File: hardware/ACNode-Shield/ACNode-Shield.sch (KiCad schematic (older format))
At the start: 15 parts, among them J1 MICRO_SD_HINGE, P1 CONN_NFC, P2 CONN_RELAY, P3 CONN_RGB_LED, P4 CONN_X6, P5 CONN_X7, P6 CONN_WS2812, Q1 PN2222A, SW1 SW_RST, SW2 SW_BTN, U1 SRD-05VDC-SL-C, U2 WS2812B

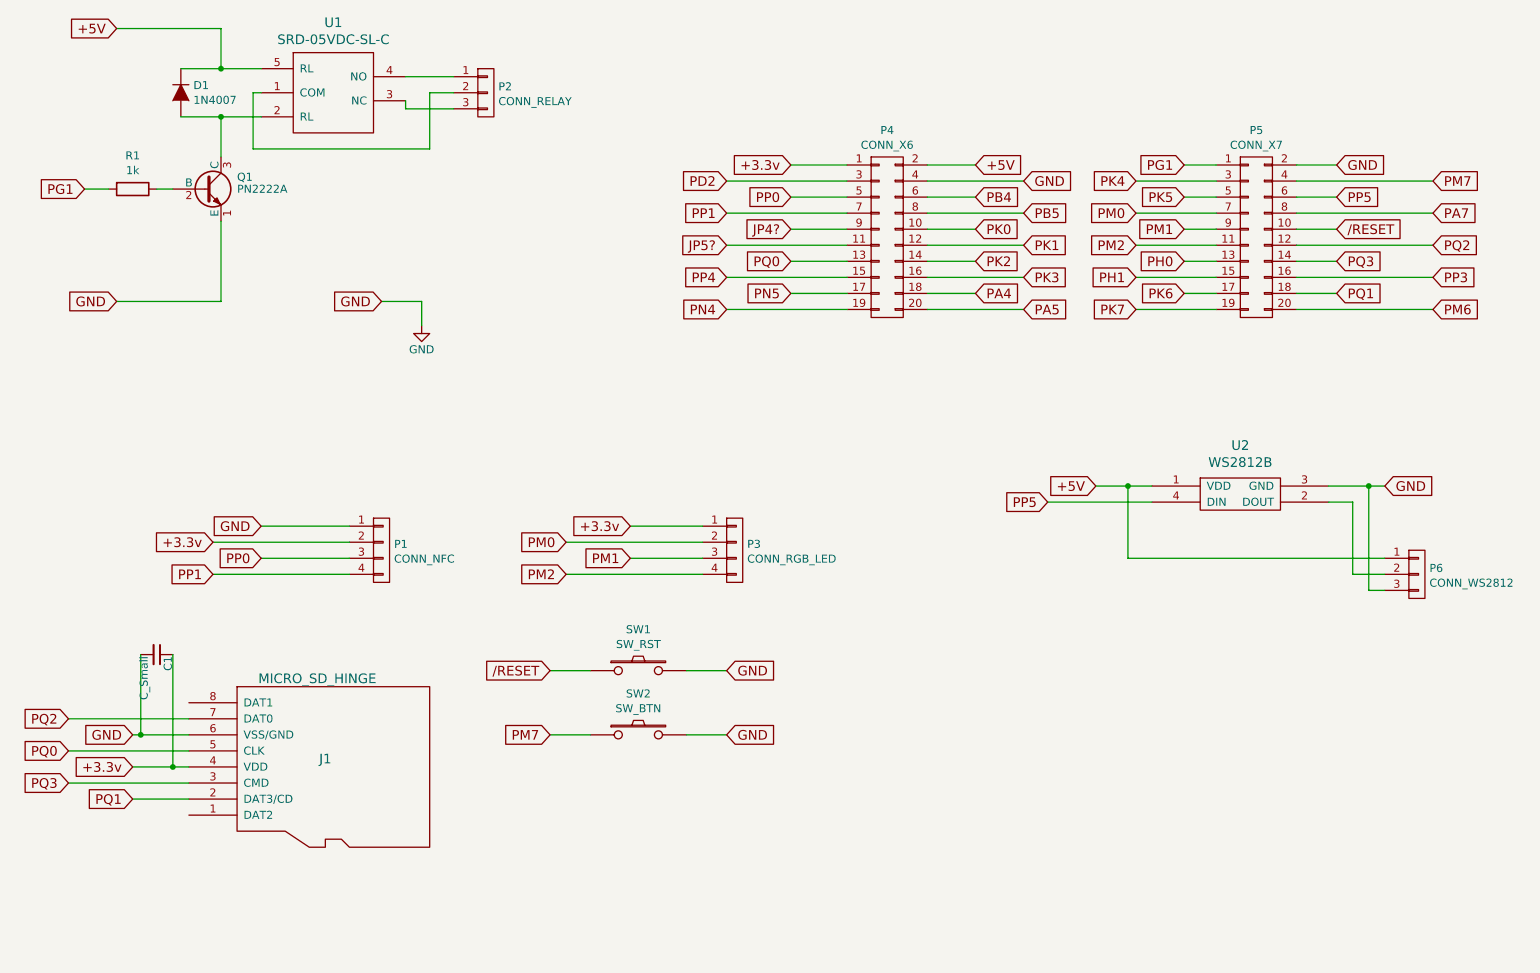
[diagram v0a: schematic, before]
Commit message: Rev 2 off to the fab
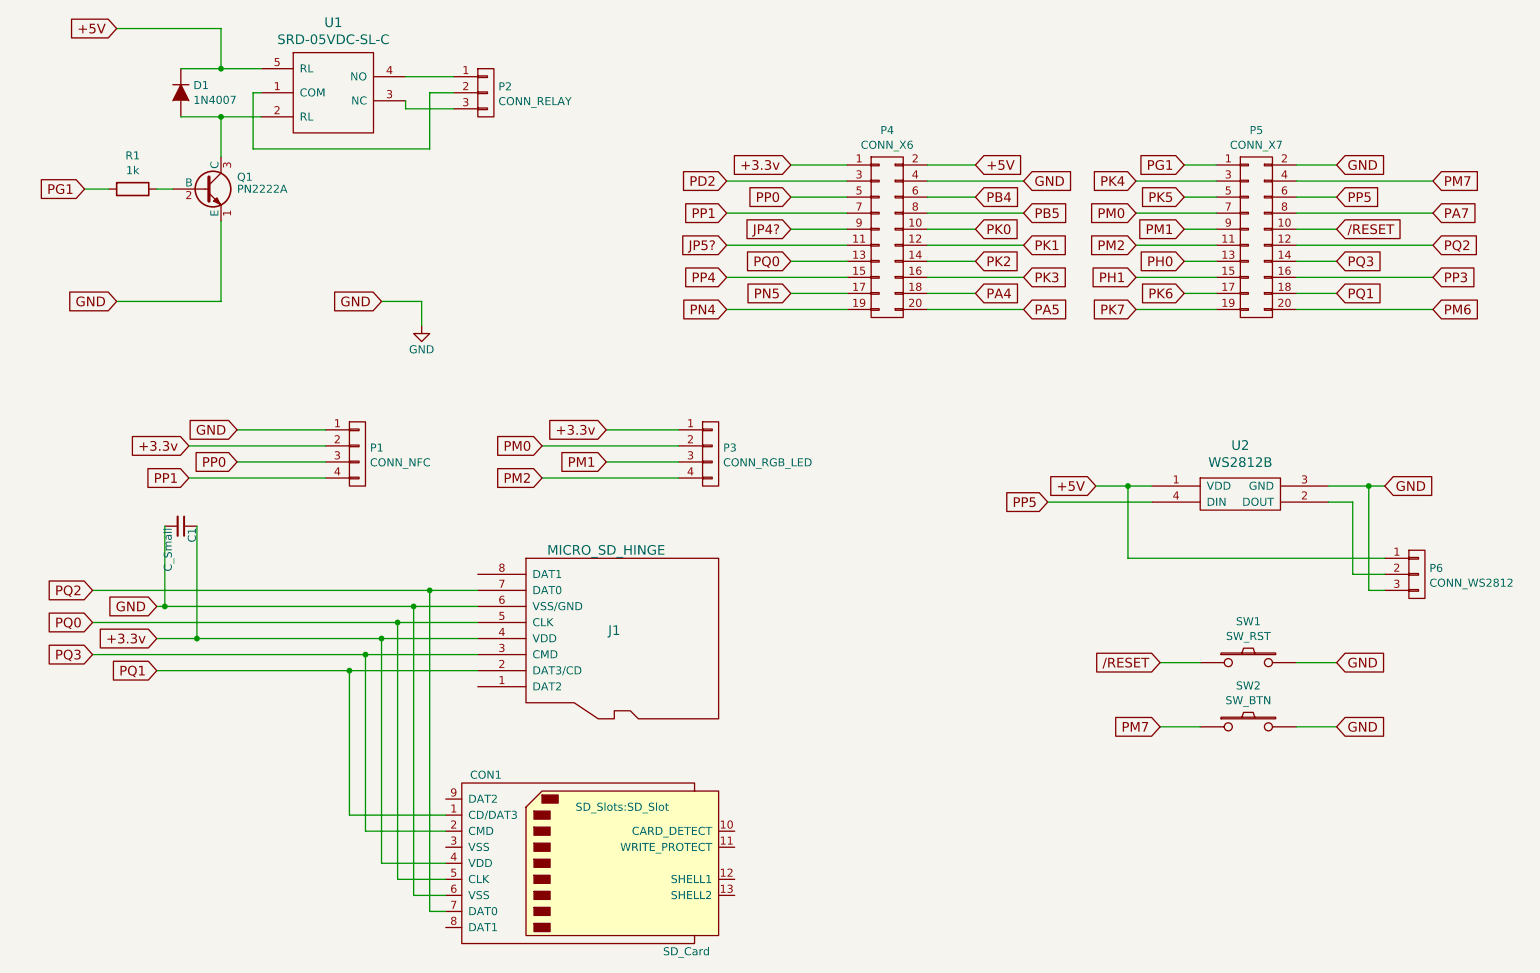
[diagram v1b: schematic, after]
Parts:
- added CON1: SD_Card, SD_Slots:SD_Slot, symbol SD_Card
- P2: footprint Pin_Headers:Pin_Header_Straight_1x03 -> Terminal_Blocks:TerminalBlock_Pheonix_MKDS1.5-3pol
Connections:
- net +3.3v: now also CON1.4 (VDD)
- net GND: now also CON1.6 (VSS)
- net PQ0: now also CON1.5 (CLK)
- net PQ1: now also CON1.1 (CD/DAT3)
- net PQ2: now also CON1.7 (DAT0)
- net PQ3: now also CON1.2 (CMD)
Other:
- moved on the sheet: C1, J1, P1, P3, SW1, SW2
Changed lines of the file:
@@
 L CONN_01X04 P1
 U 1 1 572DBA37
-P 3750 4850
-F 0 "P1" H 3828 4888 50  0000 L CNN
-F 1 "CONN_NFC" H 3828 4796 50  0000 L CNN
-F 2 "Pin_Headers:Pin_Header_Straight_1x04" H 3750 4850 50  0001 C CNN
-F 3 "" H 3750 4850 50  0000 C CNN
-	1    3750 4850
-	1    0    0    -1
-$EndComp
-Text GLabel 3000 4700 0    60   Input ~ 0
-GND
-Text GLabel 2700 4800 0    60   Input ~ 0
+P 3600 4250
+F 0 "P1" H 3678 4288 50  0000 L CNN
+F 1 "CONN_NFC" H 3678 4196 50  0000 L CNN
+F 2 "Pin_Headers:Pin_Header_Straight_1x04" H 3600 4250 50  0001 C CNN
+F 3 "" H 3600 4250 50  0000 C CNN
+	1    3600 4250
+	1    0    0    -1
+$EndComp
+Text GLabel 2850 4100 0    60   Input ~ 0
+GND
+Text GLabel 2550 4200 0    60   Input ~ 0
 +3.3v
-Text GLabel 3000 4900 0    60   Input ~ 0
+Text GLabel 2850 4300 0    60   Input ~ 0
 PP0
-Text GLabel 2700 5000 0    60   Input ~ 0
+Text GLabel 2550 4400 0    60   Input ~ 0
 PP1
 Wire Wire Line
-	3000 4700 3550 4700
-Wire Wire Line
-	3550 4800 2700 4800
-Wire Wire Line
-	3000 4900 3550 4900
-Wire Wire Line
-	3550 5000 2700 5000
+	2850 4100 3400 4100
+Wire Wire Line
+	3400 4200 2550 4200
+Wire Wire Line
+	2850 4300 3400 4300
+Wire Wire Line
+	3400 4400 2550 4400
 $Comp
 L CONN_01X04 P3
 U 1 1 572DBB8D
-P 5950 4850
-F 0 "P3" H 6028 4888 50  0000 L CNN
-F 1 "CONN_RGB_LED" H 6028 4796 50  0000 L CNN
-F 2 "Pin_Headers:Pin_Header_Straight_1x04" H 5950 4850 50  0001 C CNN
-F 3 "" H 5950 4850 50  0000 C CNN
-	1    5950 4850
-	1    0    0    -1
-$EndComp
-Text GLabel 5300 4700 0    60   Input ~ 0
+P 5800 4250
+F 0 "P3" H 5878 4288 50  0000 L CNN
+F 1 "CONN_RGB_LED" H 5878 4196 50  0000 L CNN
+F 2 "Pin_Headers:Pin_Header_Straight_1x04" H 5800 4250 50  0001 C CNN
+F 3 "" H 5800 4250 50  0000 C CNN
+	1    5800 4250
+	1    0    0    -1
+$EndComp
+Text GLabel 5150 4100 0    60   Input ~ 0
 +3.3v
-Text GLabel 4900 4800 0    60   Input ~ 0
+Text GLabel 4750 4200 0    60   Input ~ 0
 PM0
-Text GLabel 5300 4900 0    60   Input ~ 0
+Text GLabel 5150 4300 0    60   Input ~ 0
 PM1
-Text GLabel 4900 5000 0    60   Input ~ 0
+Text GLabel 4750 4400 0    60   Input ~ 0
 PM2
 Wire Wire Line
-	5300 4700 5750 4700
-Wire Wire Line
-	5750 4800 4900 4800
-Wire Wire Line
-	5300 4900 5750 4900
-Wire Wire Line
-	5750 5000 4900 5000
+	5150 4100 5600 4100
+Wire Wire Line
+	5600 4200 4750 4200
+Wire Wire Line
+	5150 4300 5600 4300
+Wire Wire Line
+	5600 4400 4750 4400
 $Comp
 L SW_PUSH SW1
 U 1 1 572DBD3B
-P 5350 5600
-F 0 "SW1" H 5350 5856 50  0000 C CNN
-F 1 "SW_RST" H 5350 5764 50  0000 C CNN
-F 2 "Buttons_Switches_ThroughHole:SW_PUSH_SMALL" H 5350 5600 50  0001 C CNN
-F 3 "" H 5350 5600 50  0000 C CNN
-	1    5350 5600
-	1    0    0    -1
-$EndComp
-Text GLabel 4800 5600 0    60   Input ~ 0
+P 9150 5550
+F 0 "SW1" H 9150 5806 50  0000 C CNN
+F 1 "SW_RST" H 9150 5714 50  0000 C CNN
+F 2 "Buttons_Switches_ThroughHole:SW_PUSH_SMALL" H 9150 5550 50  0001 C CNN
+F 3 "" H 9150 5550 50  0000 C CNN
+	1    9150 5550
+	1    0    0    -1
+$EndComp
+Text GLabel 8600 5550 0    60   Input ~ 0
 /RESET
-Text GLabel 5900 5600 2    60   Input ~ 0
-GND
-Wire Wire Line
-	5650 5600 5900 5600
-Wire Wire Line
-	5050 5600 4800 5600
+Text GLabel 9700 5550 2    60   Input ~ 0
+GND
+Wire Wire Line
+	9450 5550 9700 5550
+Wire Wire Line
+	8850 5550 8600 5550
 $Comp
 L WS2812B U2
@@
 L SW_PUSH SW2
 U 1 1 572DC67E
-P 5350 6000
-F 0 "SW2" H 5350 6256 50  0000 C CNN
-F 1 "SW_BTN" H 5350 6164 50  0000 C CNN
-F 2 "Socket_Strips:Socket_Strip_Straight_1x02" H 5350 6000 50  0001 C CNN
-F 3 "" H 5350 6000 50  0000 C CNN
-	1    5350 6000
-	1    0    0    -1
-$EndComp
-Text GLabel 5900 6000 2    60   Input ~ 0
-GND
-Text GLabel 4800 6000 0    60   Input ~ 0
+P 9150 5950
+F 0 "SW2" H 9150 6206 50  0000 C CNN
+F 1 "SW_BTN" H 9150 6114 50  0000 C CNN
+F 2 "Socket_Strips:Socket_Strip_Straight_1x02" H 9150 5950 50  0001 C CNN
+F 3 "" H 9150 5950 50  0000 C CNN
+	1    9150 5950
+	1    0    0    -1
+$EndComp
+Text GLabel 9700 5950 2    60   Input ~ 0
+GND
+Text GLabel 8600 5950 0    60   Input ~ 0
 PM7
 Wire Wire Line
-	4800 6000 5050 6000
-Wire Wire Line
-	5650 6000 5900 6000
+	8600 5950 8850 5950
+Wire Wire Line
+	9450 5950 9700 5950
 $Comp
 L SRD-05VDC-SL-C U1
@@
 F 0 "P2" H 4478 2038 50  0000 L CNN
 F 1 "CONN_RELAY" H 4478 1946 50  0000 L CNN
-F 2 "Pin_Headers:Pin_Header_Straight_1x03" H 4400 2000 50  0001 C CNN
+F 2 "Terminal_Blocks:TerminalBlock_Pheonix_MKDS1.5-3pol" H 4400 2000 50  0001 C CNN
 F 3 "" H 4400 2000 50  0000 C CNN
 	1    4400 2000
@@
 L MICRO_SD_HINGE J1
 U 1 1 572E391C
-P 3350 6200
-F 0 "J1" H 3400 6250 60  0000 C CNN
-F 1 "MICRO_SD_HINGE" H 3350 6750 60  0000 C CNN
-F 2 "SD_Slots:MicroSD_Slot" V 3460 5700 60  0001 C CNN
-F 3 "" V 3460 5700 60  0000 C CNN
-	1    3350 6200
-	1    0    0    -1
-$EndComp
-Text GLabel 2200 6400 0    60   Input ~ 0
+P 5150 5400
+F 0 "J1" H 5200 5450 60  0000 C CNN
+F 1 "MICRO_SD_HINGE" H 5150 5950 60  0000 C CNN
+F 2 "SD_Slots:MicroSD_Slot" V 5260 4900 60  0001 C CNN
+F 3 "" V 5260 4900 60  0000 C CNN
+	1    5150 5400
+	1    0    0    -1
+$EndComp
+Text GLabel 2350 5600 0    60   Input ~ 0
 PQ1
-Text GLabel 1800 6300 0    60   Input ~ 0
+Text GLabel 1950 5500 0    60   Input ~ 0
 PQ3
-Text GLabel 2200 6200 0    60   Input ~ 0
+Text GLabel 2350 5400 0    60   Input ~ 0
 +3.3v
-Text GLabel 1800 6100 0    60   Input ~ 0
+Text GLabel 1950 5300 0    60   Input ~ 0
 PQ0
-Text GLabel 2200 6000 0    60   Input ~ 0
-GND
-Text GLabel 1800 5900 0    60   Input ~ 0
+Text GLabel 2350 5200 0    60   Input ~ 0
+GND
+Text GLabel 1950 5100 0    60   Input ~ 0
 PQ2
 Wire Wire Line
-	2200 6400 2550 6400
-Wire Wire Line
-	2550 6300 1800 6300
-Wire Wire Line
-	2200 6200 2550 6200
-Wire Wire Line
-	1800 6100 2550 6100
-Wire Wire Line
-	2550 6000 2200 6000
-Wire Wire Line
-	1800 5900 2550 5900
+	2350 5600 4350 5600
+Wire Wire Line
+	1950 5500 4350 5500
+Wire Wire Line
+	2350 5400 4350 5400
+Wire Wire Line
+	1950 5300 4350 5300
+Wire Wire Line
+	2350 5200 4350 5200
+Wire Wire Line
+	1950 5100 4350 5100
 $Comp
 L C_Small C1
 U 1 1 5736F818
-P 2350 5500
-F 0 "C1" H 2360 5570 50  0000 L CNN
-F 1 "C_Small" H 2360 5420 50  0000 L CNN
-F 2 "Capacitors_SMD:C_1206" H 2350 5500 50  0001 C CNN
-F 3 "" H 2350 5500 50  0000 C CNN
-	1    2350 5500
+P 2500 4700
+F 0 "C1" H 2510 4770 50  0000 L CNN
+F 1 "C_Small" H 2510 4620 50  0000 L CNN
+F 2 "Capacitors_SMD:C_1206" H 2500 4700 50  0001 C CNN
+F 3 "" H 2500 4700 50  0000 C CNN
+	1    2500 4700
 	0    1    1    0
 $EndComp
 Wire Wire Line
-	2250 5500 2250 6000
-Connection ~ 2250 6000
-Wire Wire Line
-	2450 5500 2450 6200
-Connection ~ 2450 6200
+	2400 4700 2400 5200
+Connection ~ 2400 5200
+Wire Wire Line
+	2600 4700 2600 5400
+Connection ~ 2600 5400
+$Comp
+L SD_Card CON1
+U 1 1 57ED844B
+P 5050 6800
+F 0 "CON1" H 4400 7350 50  0000 C CNN
+F 1 "SD_Card" H 5650 6250 50  0000 C CNN
+F 2 "SD_Slots:SD_Slot" H 5250 7150 50  0000 C CNN
+F 3 "" H 5050 6800 50  0000 C CNN
+	1    5050 6800
+	1    0    0    -1
+$EndComp
+Wire Wire Line
+	4150 7100 4050 7100
+Wire Wire Line
+	4050 7100 4050 5100
+Connection ~ 4050 5100
+Wire Wire Line
+	4150 7000 3950 7000
+Wire Wire Line
+	3950 7000 3950 5200
+Connection ~ 3950 5200
+Wire Wire Line
+	4150 6900 3850 6900
+Wire Wire Line
+	3850 6900 3850 5300
+Connection ~ 3850 5300
+Wire Wire Line
+	4150 6800 3750 6800
+Wire Wire Line
+	3750 6800 3750 5400
+Connection ~ 3750 5400
+Wire Wire Line
+	4150 6600 3650 6600
+Wire Wire Line
+	3650 6600 3650 5500
+Connection ~ 3650 5500
+Wire Wire Line
+	4150 6500 3550 6500
+Wire Wire Line
+	3550 6500 3550 5600
+Connection ~ 3550 5600
 $EndSCHEMATC
